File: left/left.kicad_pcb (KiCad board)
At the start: 2 copper layers, 143.8 x 147.7 mm, 45 parts, among them J1 USB_C_Receptacle_USB2.0, J2 Conn_01x04, SW1 SW_Push, SW10 SW_Push, SW11 SW_Push, SW12 SW_Push, SW13 SW_Push, SW14 SW_Push, SW15 SW_Push, SW16 SW_Push, SW17 SW_Push, SW18 SW_Push, SW19 SW_Push, SW2 SW_Push, SW20 SW_Push, SW21 SW_Push, SW22 SW_Push, SW23 SW_Push, SW24 SW_Push, SW25 SW_Push, SW26 SW_Push, SW27 SW_Push, SW28 SW_Push, SW29 SW_Push, SW3 RotaryEncoder_Switch, SW30 SW_Push, SW31 SW_Push, SW32 SW_Push, SW33 SW_Push, SW34 SW_Push, SW4 SW_Push, SW5 SW_Push, SW6 SW_Push, SW7 SW_Push, SW8 SW_Push, SW9 SW_Push, U1 HOLYIOT-18010-NRF52840

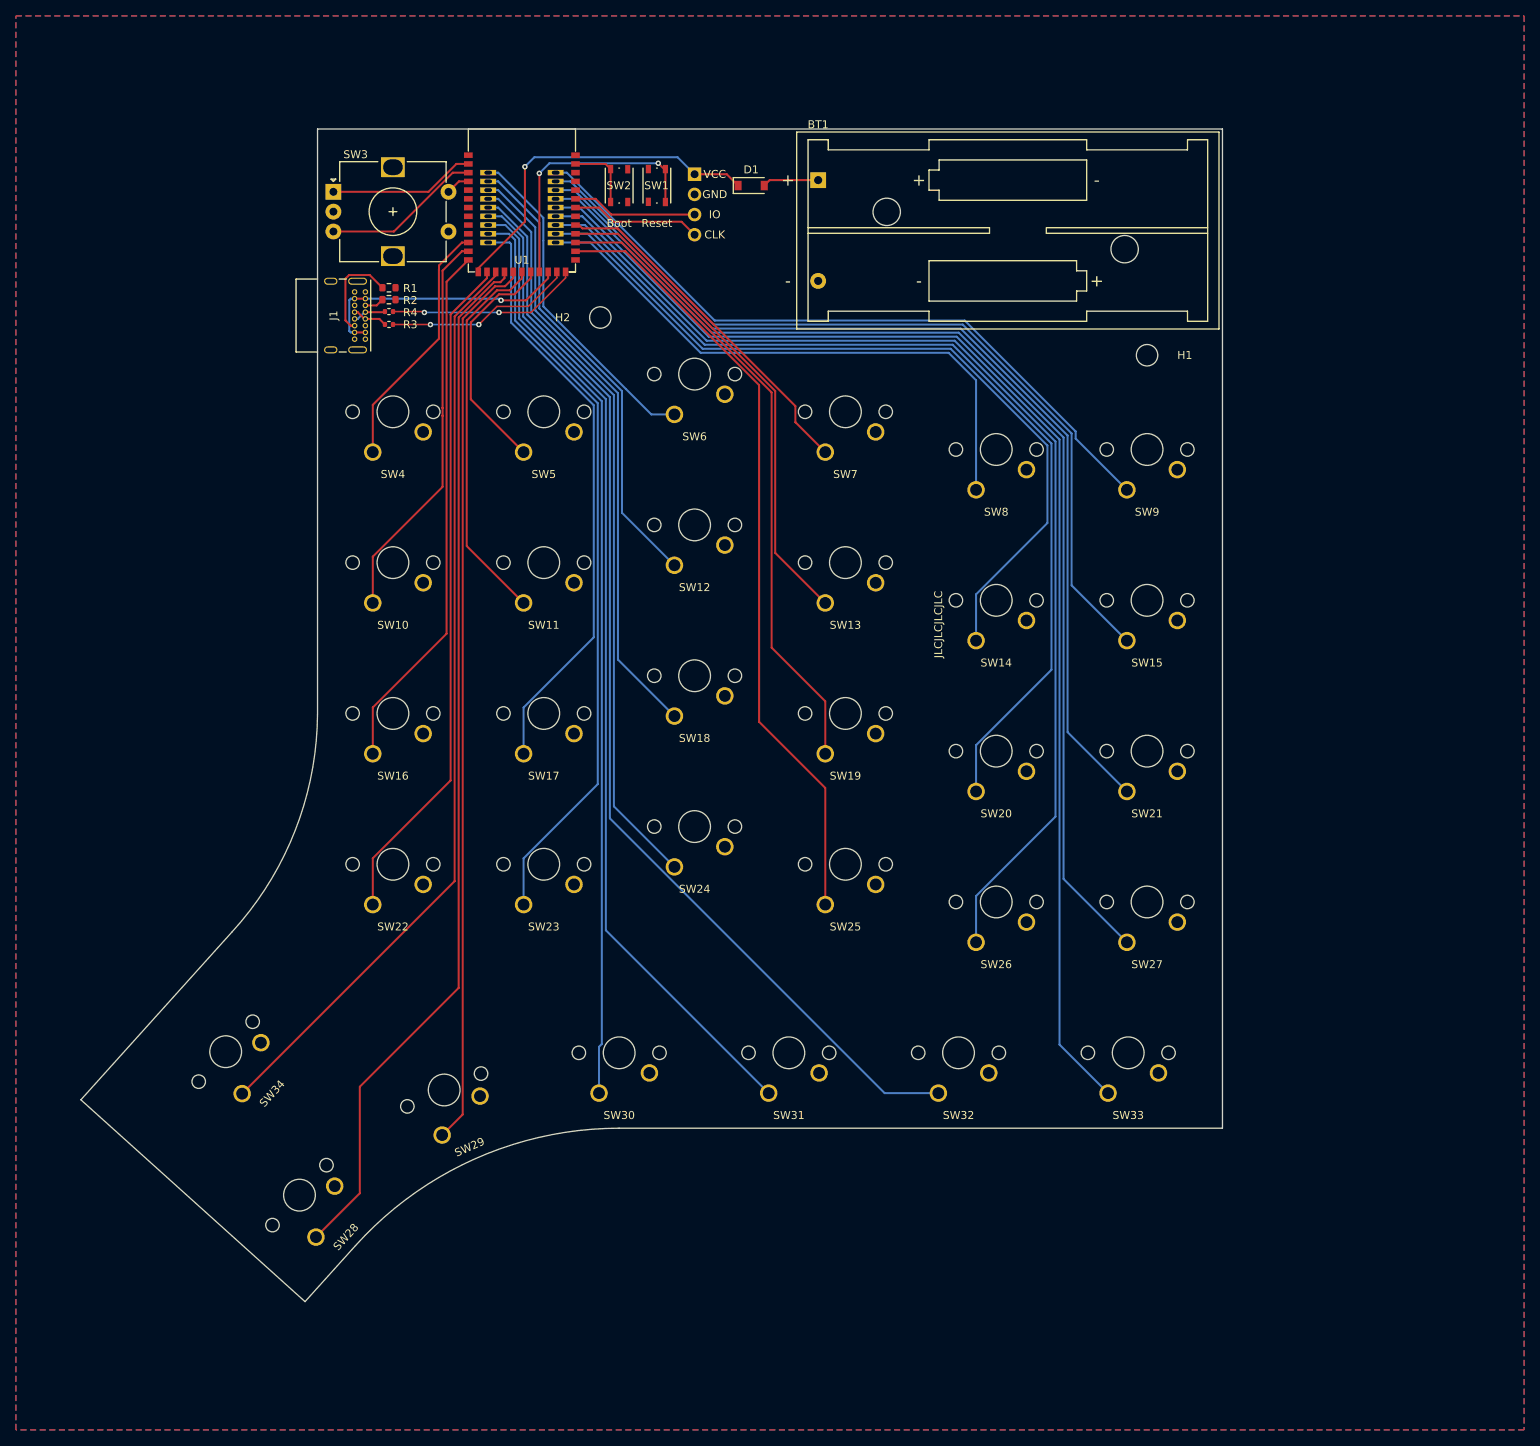
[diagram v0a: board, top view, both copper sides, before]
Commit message: right finished, left wip
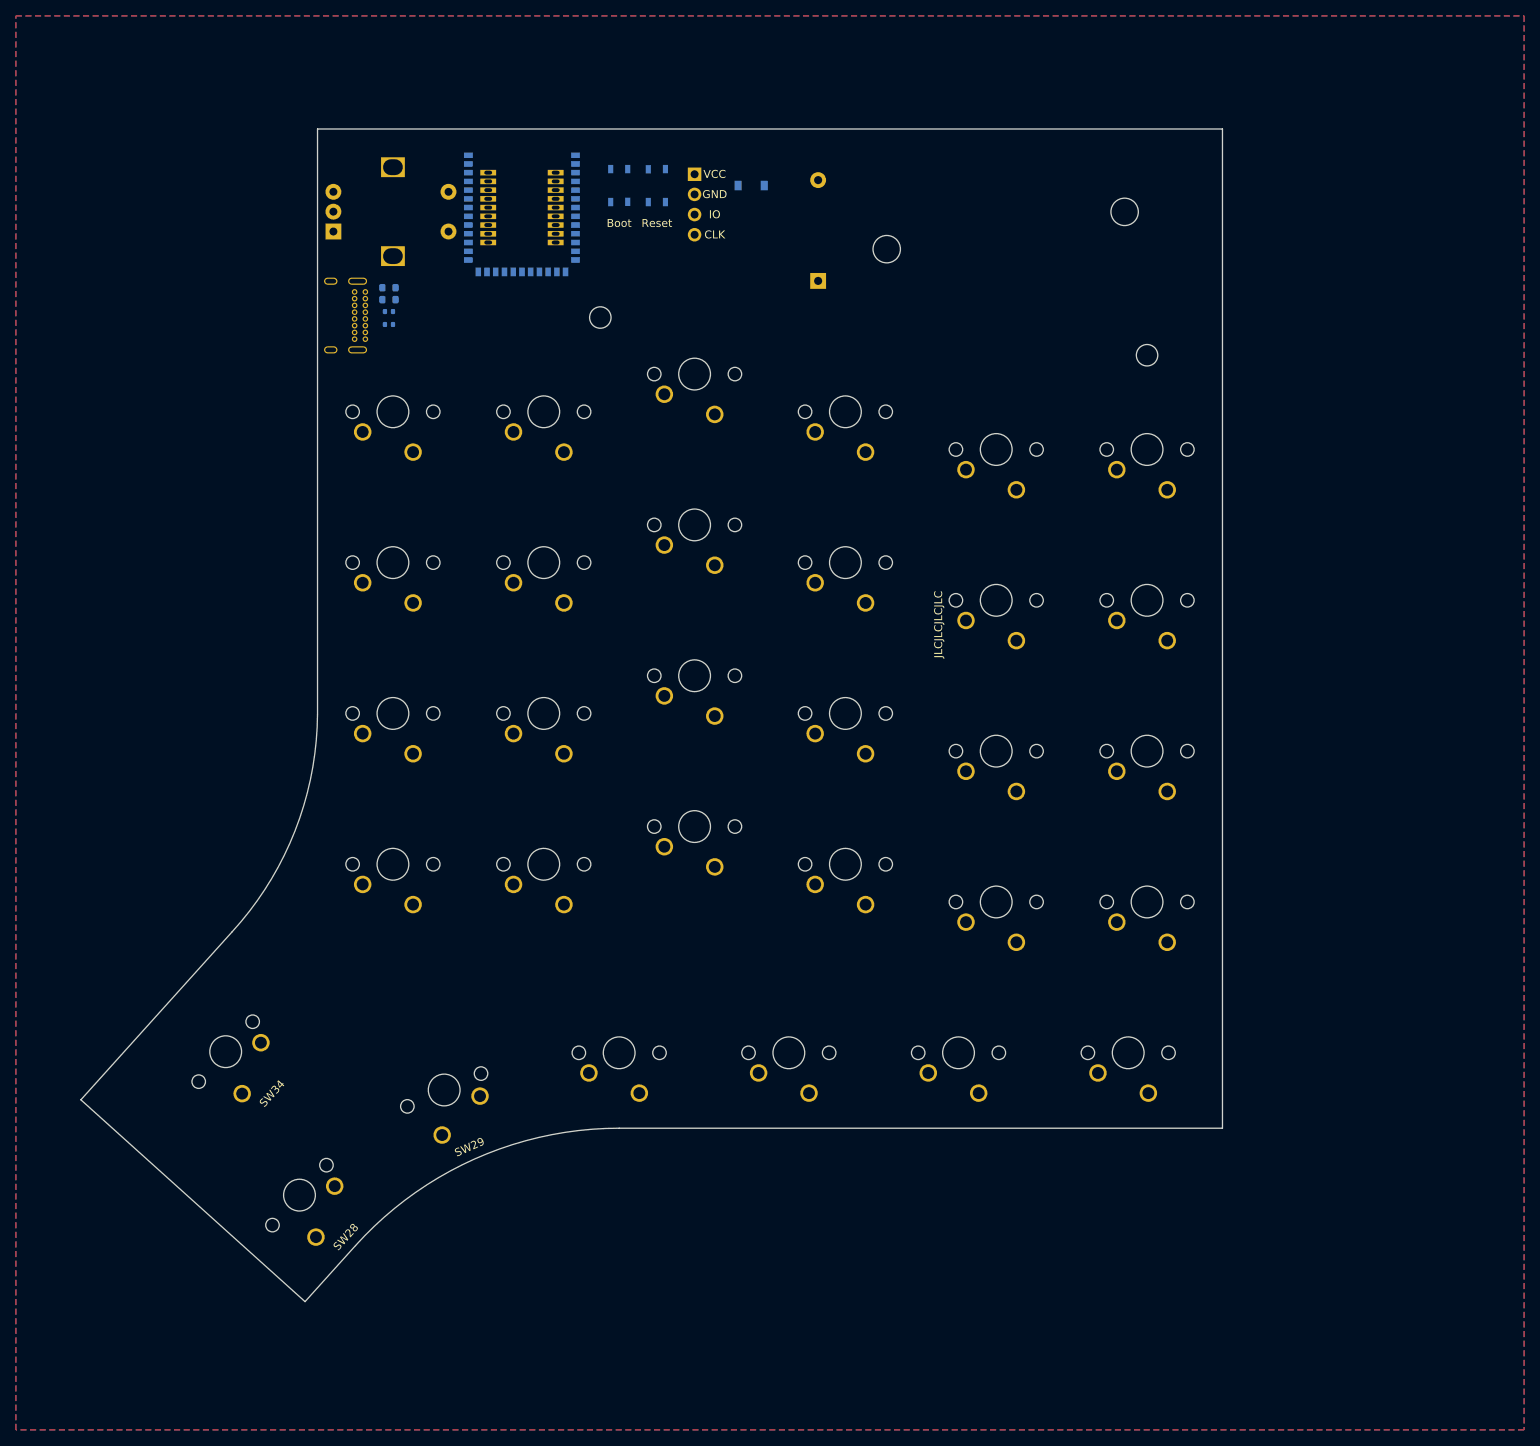
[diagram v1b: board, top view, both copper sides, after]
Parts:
- BT1, D1, H1, H2, J1, J2, R1, R2, R3, R4, SW1, SW10, SW11, SW12, SW13, SW14, SW15, SW16, SW17, SW18, SW19, SW2, SW20, SW21, SW22, SW23, SW24, SW25, SW26, SW27, SW3, SW30, SW31, SW32, SW33, SW4, SW5, SW6, SW7, SW8, SW9, U1: moved to B.Cu
- moved U1 13.5 mm to (112.4, 19.0), turned to 180 degrees
- moved BT1 12.7 mm to (143.0, 38.1)
- moved J1 5.95 mm to (85.9, 45.5), turned to 90 degrees
- moved SW12 5.08 mm to (129.9, 74.0), turned to 0 degrees
- moved SW13 5.08 mm to (148.9, 78.7), turned to 0 degrees
- moved SW14 5.08 mm to (167.9, 83.5), turned to 0 degrees
- moved SW15 5.08 mm to (186.9, 83.5), turned to 0 degrees
- moved SW19 5.08 mm to (148.9, 97.7), turned to 0 degrees
- moved SW20 5.08 mm to (167.9, 102.5), turned to 0 degrees
- moved SW25 5.08 mm to (148.9, 116.7), turned to 0 degrees
- moved SW31 5.08 mm to (141.8, 140.5), turned to 0 degrees
- moved SW33 5.08 mm to (184.6, 140.5), turned to 0 degrees
- moved SW8 5.08 mm to (167.9, 64.5), turned to 0 degrees
- moved SW10 5.08 mm to (91.9, 78.7), turned to 0 degrees
- moved SW11 5.08 mm to (110.9, 78.7), turned to 0 degrees
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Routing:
- net S45: track 160.4 -> 0.00 mm
- net S35: track 143.3 -> 0.00 mm
- net S34: track 141.9 -> 0.00 mm
- net S44: track 139.7 -> 0.00 mm
- net S40: track 131.9 -> 0.00 mm
- net S43: track 126.1 -> 0.00 mm
- net S25: track 125.2 -> 0.00 mm
- net S24: track 121.6 -> 0.00 mm
- net S50: track 116.8 -> 0.00 mm
- net S42: track 116.7 -> 0.00 mm
- net S41: track 113.2 -> 0.00 mm
- net S15: track 107.1 -> 0.00 mm
- net S14: track 101.3 -> 0.00 mm
- net S33: track 99.0 -> 0.00 mm
- net S31: track 95.6 -> 0.00 mm
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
